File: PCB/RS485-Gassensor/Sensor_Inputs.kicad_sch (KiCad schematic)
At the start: 31 parts, among them J8 Conn_01x03, J9 Conn_01x03, SW1 SW_DIP_x06, U3 MCP6002-xMS, U6 MCP6002-xMS

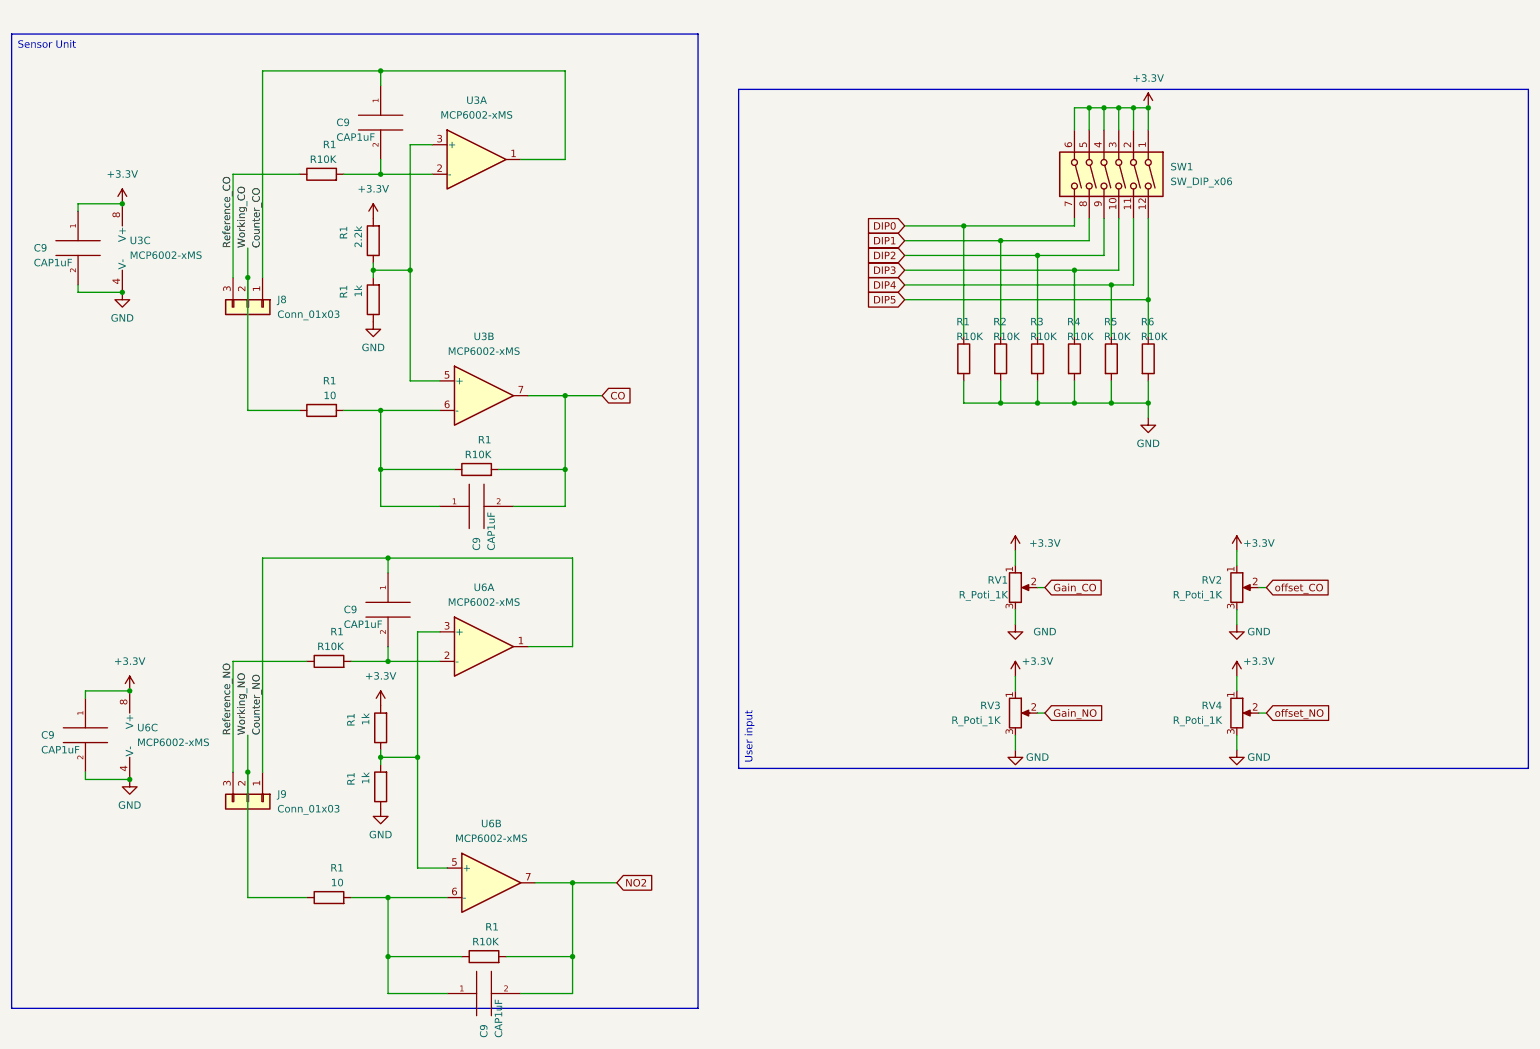
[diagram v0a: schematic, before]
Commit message: made For NAP505 and NAP550
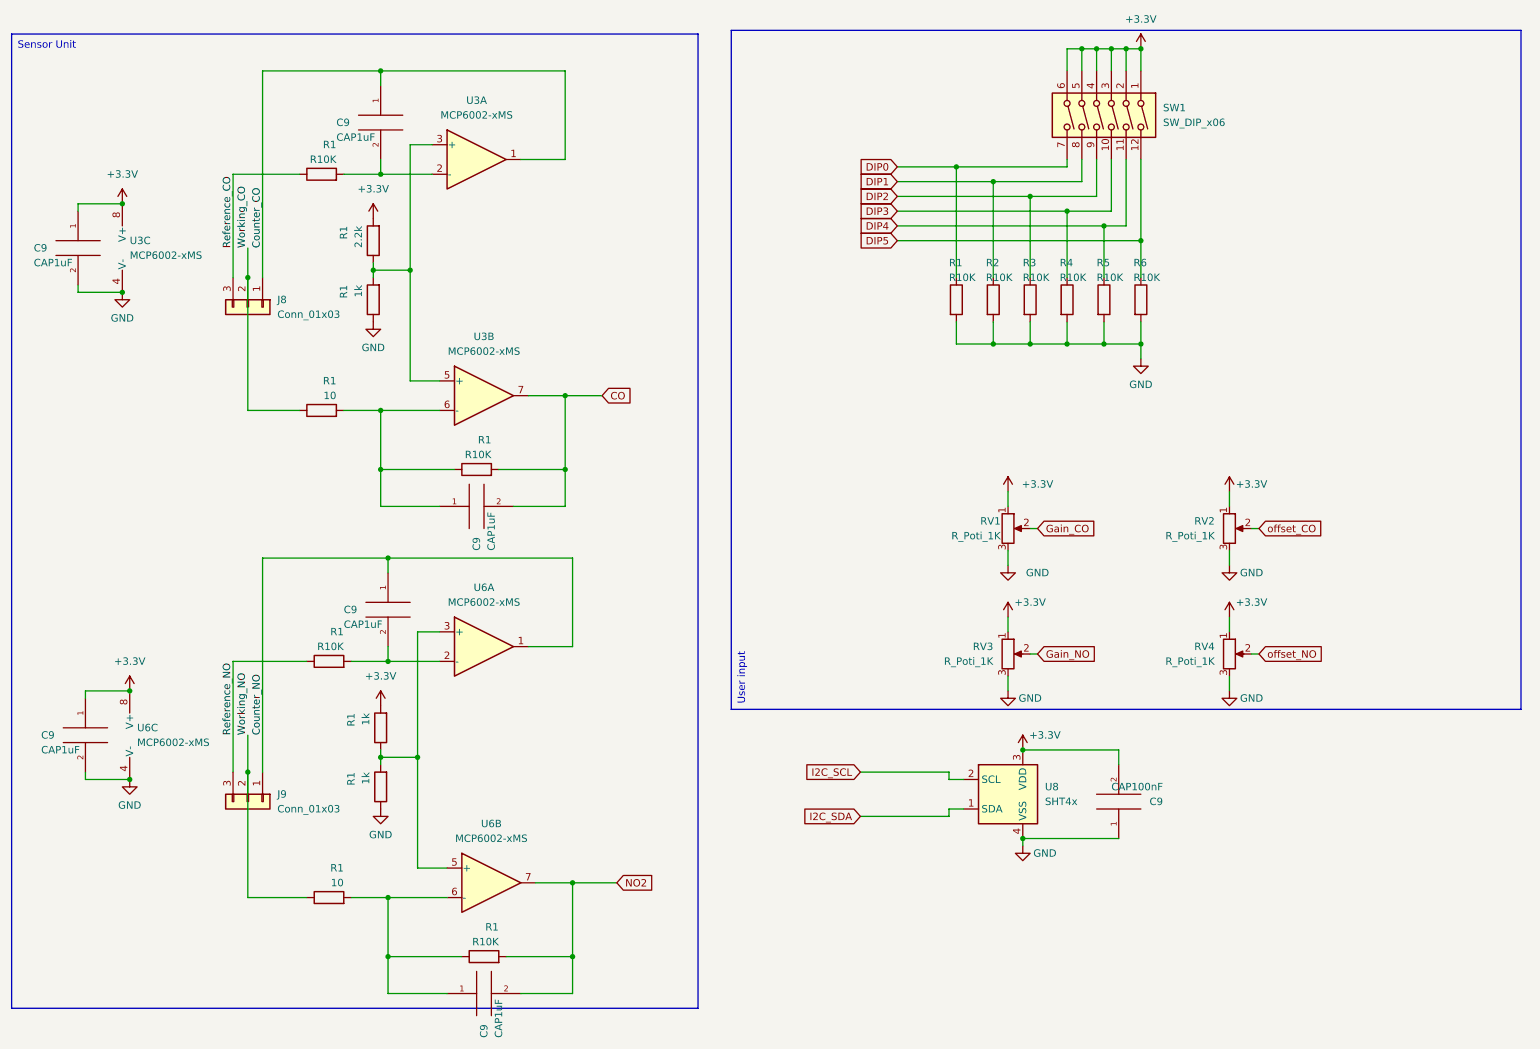
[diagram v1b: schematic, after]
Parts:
- added C9: CAP100nF, Capacitor_SMD:C_0603_1608Metric, symbol pspice:CAP
- added U8: SHT4x, Sensor_Humidity:Sensirion_DFN-4_1.5x1.5mm_P0.8mm_SHT4x_NoCentralPad, symbol Sensor_Humidity:SHT4x
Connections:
- net +3.3V: now also C9.2, U8.3 (VDD)
- net GND: now also C9.1, U8.4 (VSS)
- new net I2C_SCL: U8.2 (SCL)
- new net I2C_SDA: U8.1 (SDA)
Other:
- moved on the sheet: R1, R2, R3, R4, R5, R6, RV1, RV2, RV3, RV4, SW1
